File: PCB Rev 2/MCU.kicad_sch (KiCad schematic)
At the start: 51 parts, among them J1 USB_C_Receptacle_USB2.0_16P, J2 Conn_ARM_SWD_TagConnect_TC2030, U2 NCP718xSN330, U3 RP2354B, U7 MX25L3233FM1, Y1 Abracon ABM8-272-T3

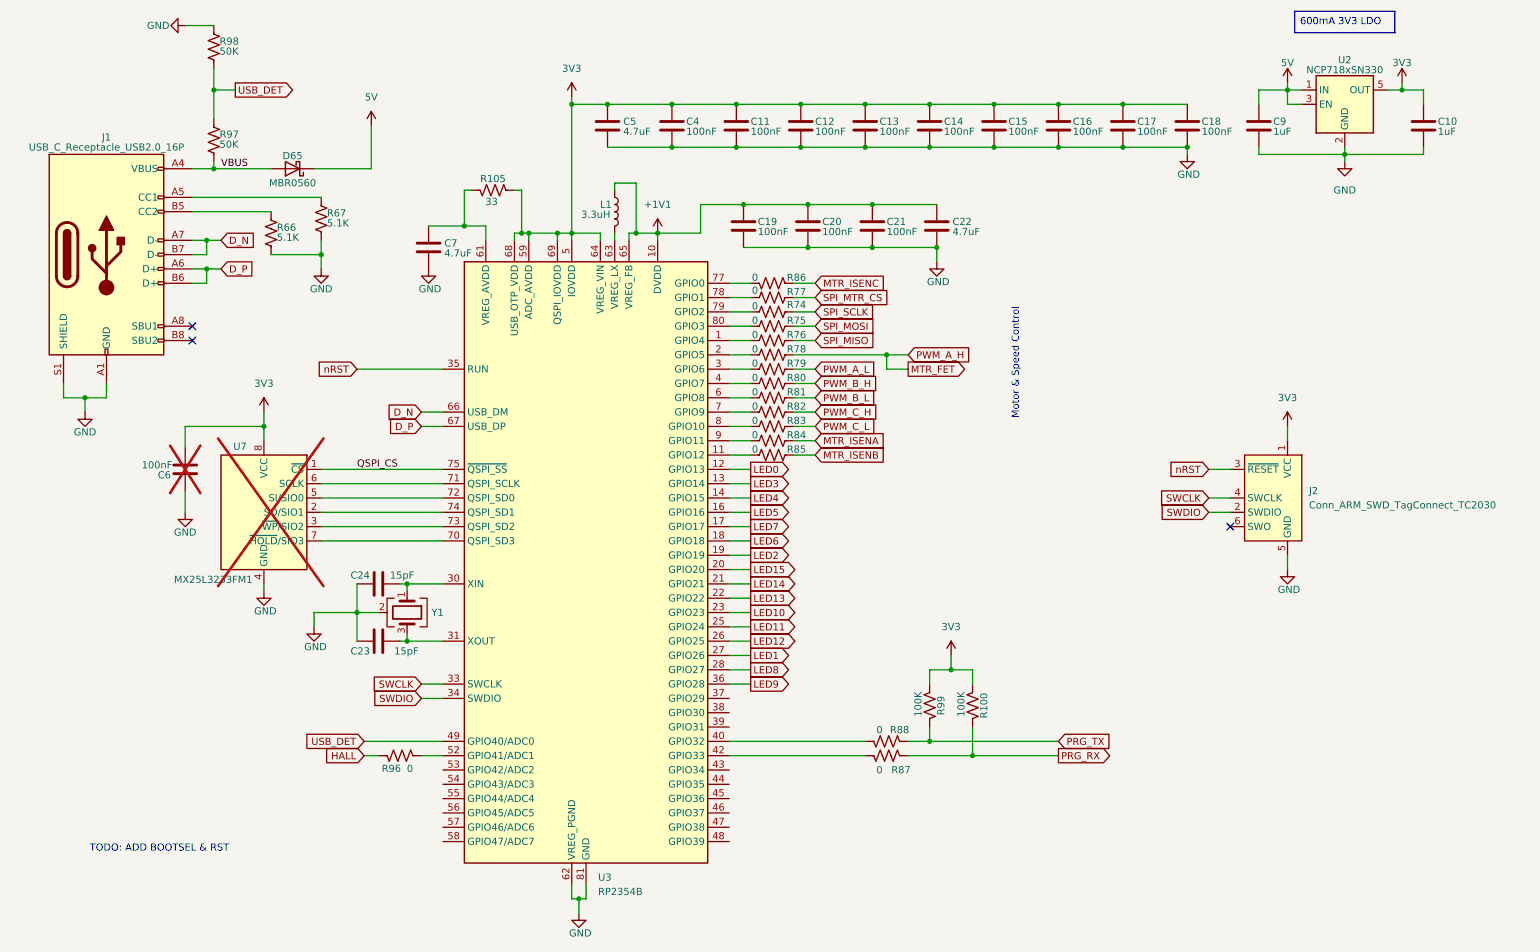
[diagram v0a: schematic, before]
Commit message: started routing rev2
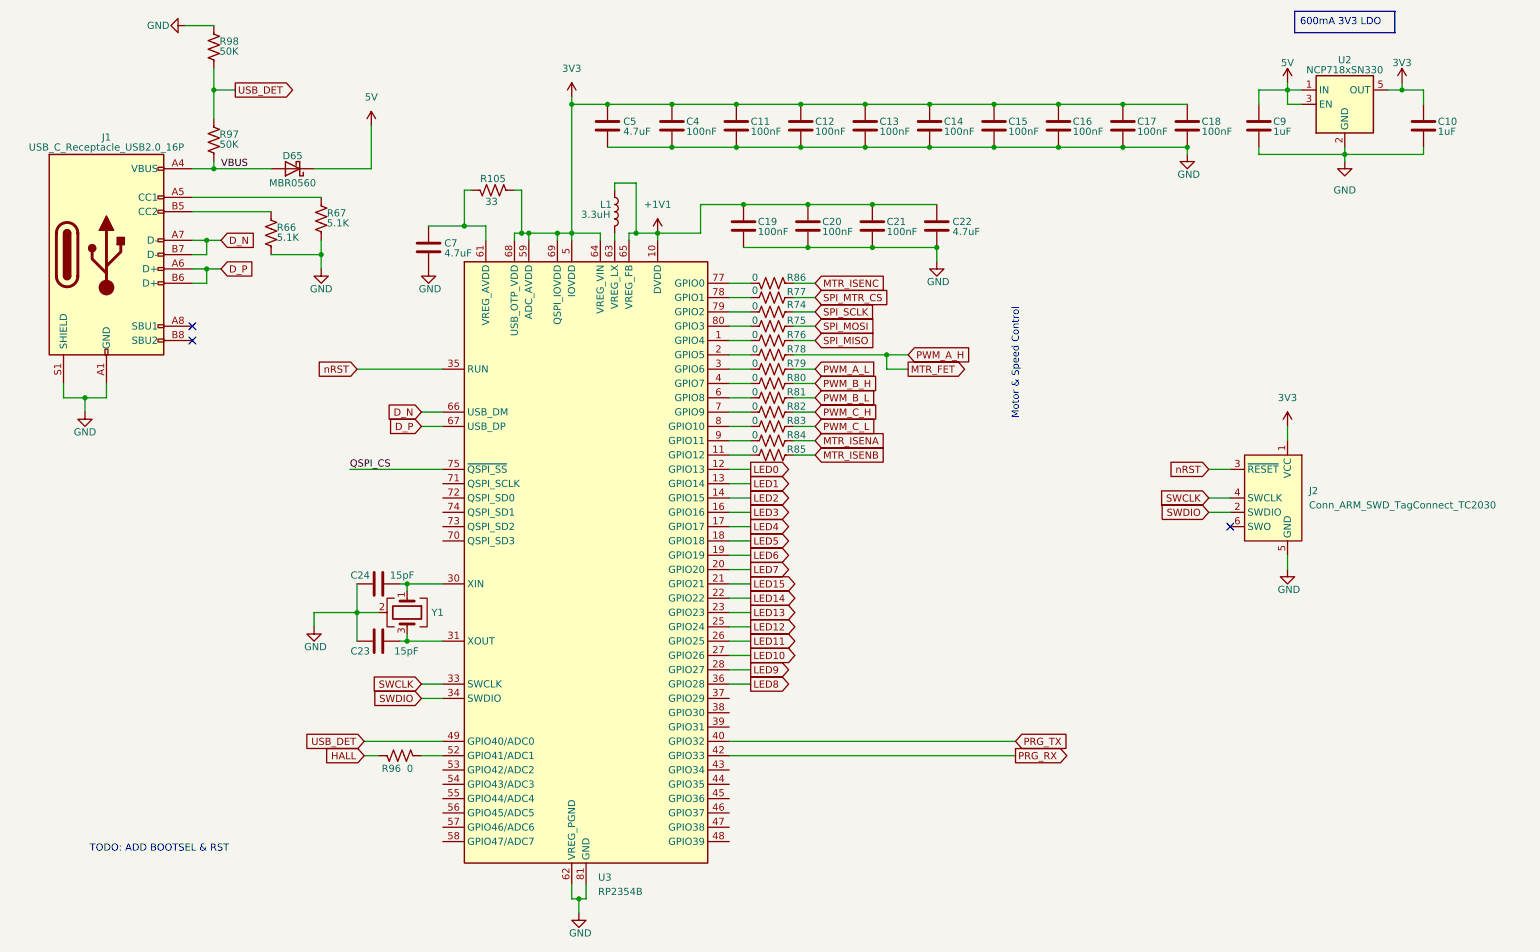
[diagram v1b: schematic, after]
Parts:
- removed C6: 100nF, Capacitor_SMD:C_0402_1005Metric_Pad0.74x0.62mm_HandSolder, symbol Device:C
- removed R100, R99: 100K, Resistor_SMD:R_0603_1608Metric_Pad0.98x0.95mm_HandSolder, symbol Device:R_US
- removed R87, R88: 0, Resistor_SMD:R_0603_1608Metric_Pad0.98x0.95mm_HandSolder, symbol Device:R_US
- removed U7: MX25L3233FM1, Package_SO:JEITA_SOIC-8_3.9x4.9mm_P1.27mm, symbol Memory_Flash:MX25L3233FM1
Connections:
- net LED1: now also U3.13 (GPIO14); no longer U3.27 (GPIO26)
- net LED10: now also U3.27 (GPIO26); no longer U3.23 (GPIO23)
- net LED11: now also U3.26 (GPIO25); no longer U3.25 (GPIO24)
- net LED12: now also U3.25 (GPIO24); no longer U3.26 (GPIO25)
- net LED13: now also U3.23 (GPIO23); no longer U3.22 (GPIO22)
- net LED14: now also U3.22 (GPIO22); no longer U3.21 (GPIO21)
- net LED15: now also U3.21 (GPIO21); no longer U3.20 (GPIO20)
- net LED2: now also U3.14 (GPIO15); no longer U3.19 (GPIO19)
- net LED3: now also U3.16 (GPIO16); no longer U3.13 (GPIO14)
- net LED4: now also U3.17 (GPIO17); no longer U3.14 (GPIO15)
- net LED5: now also U3.18 (GPIO18); no longer U3.16 (GPIO16)
- net LED6: now also U3.19 (GPIO19); no longer U3.18 (GPIO18)
- net LED7: now also U3.20 (GPIO20); no longer U3.17 (GPIO17)
- net LED8: now also U3.36 (GPIO28); no longer U3.28 (GPIO27)
- net LED9: now also U3.28 (GPIO27); no longer U3.36 (GPIO28)
- net PRG_RX: now also U3.42 (GPIO33)
- net PRG_TX: now also U3.40 (GPIO32)
